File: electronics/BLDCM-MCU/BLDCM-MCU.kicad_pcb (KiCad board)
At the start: 4 copper layers, 32 x 32 mm, 91 parts, among them J1 52991-0308, K1 EVPAKE31A, U1 STM32F446RE, U10 SK6805, U11 SK6805, U12 SK6805, U13 SK6805, U14 SK6805, U15 SK6805, U16 SK6805, U17 SK6805, U18 SK6805, U19 SK6805, U2 SN74LV1T34DBVR, U20 AS5048A, U3 ISM330DHCX, U4 SK6805, U5 SK6805, U6 SK6805, U7 SK6805, U8 SK6805, U9 SK6805, Y1 ECS-3225MVLC-240-CN

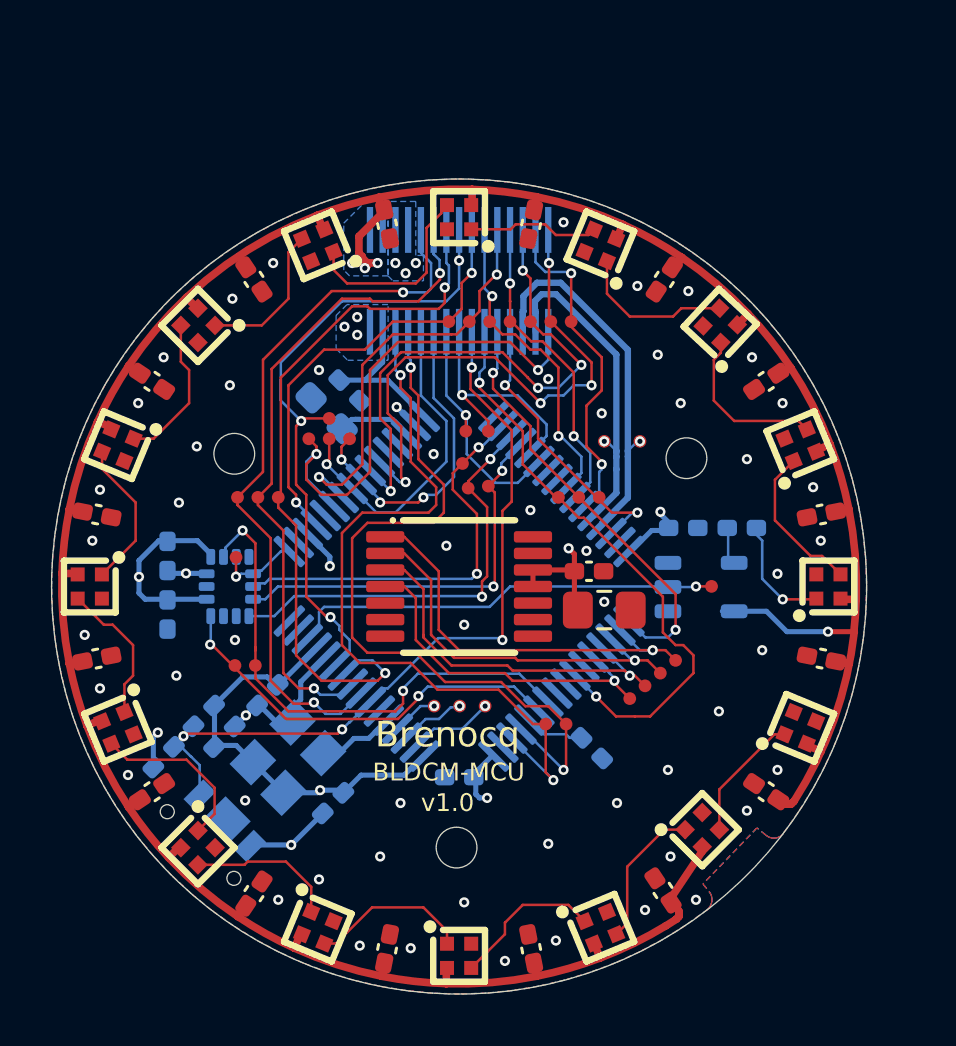
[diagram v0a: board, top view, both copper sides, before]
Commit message: Feat: PCB adjustments for manufacturing
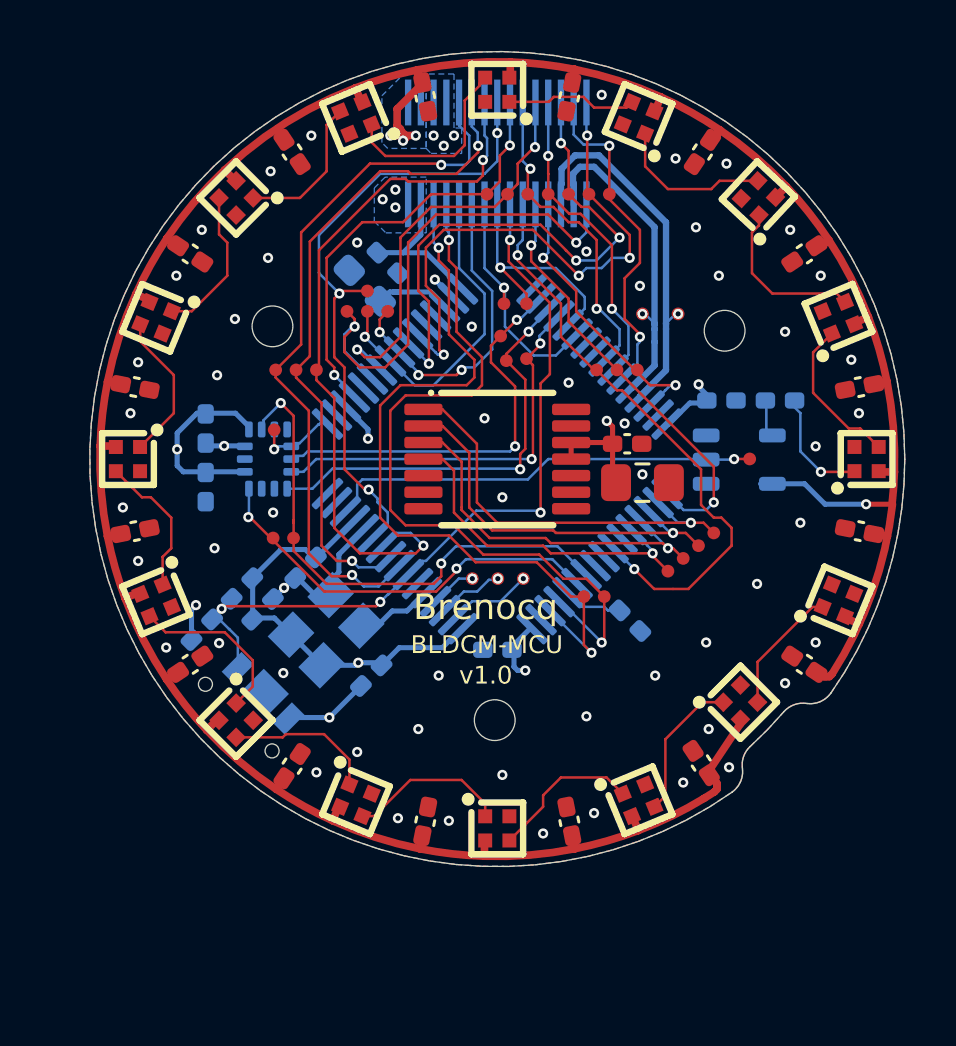
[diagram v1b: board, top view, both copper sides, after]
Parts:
- moved TP14 5.22 mm to (150.3, 93.9)
- moved TP12 5.22 mm to (151.1, 93.9)
- moved Y1 5.22 mm to (143.3, 106.7)
- moved C13 5.22 mm to (158.1, 87.9)
- moved C16 5.22 mm to (141.9, 87.9)
- moved C17 5.22 mm to (137.9, 91.9)
- moved C20 5.22 mm to (137.9, 108.1)
- moved C21 5.22 mm to (141.9, 112.1)
- moved C28 5.22 mm to (155.7, 100.9)
- moved C3 5.22 mm to (145.7, 92.3)
- moved C5 5.22 mm to (158.8, 97.7)
- moved C6 5.22 mm to (144.8, 93.2)
- moved R1 5.22 mm to (155.2, 106.3)
- moved TP11 5.22 mm to (145.7, 94.2)
- moved TP16 5.22 mm to (154.2, 105.4)
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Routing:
- net GND: vias 62 -> 63
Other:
- outline, holes or cut-outs redrawn
- rule pad_to_mask_clearance: 0.075 -> 0.05
